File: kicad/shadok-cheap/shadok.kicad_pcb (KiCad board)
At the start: 2 copper layers, 141.2 x 57.8 mm, 123 parts, among them J101 TEST_1P, J103 TEST_1P, J104 TEST_1P, J105 SERIALS, J401 Conn_02x05_Odd_Even, J501 Micro_SD_Card, J502 TEST_1P, J601 74LVC8T245, J602 74LVC8T245, J603 74LVC8T245, J604 SNP34-90, J605 74LVC8T245, J701 DB9_Male_MountingHoles, J702 DB9_Male_MountingHoles, J801 Conn_01x02, J815 Audio Out, SW101 SW_Push, U201 ADP2108-1.2, U202 LP2985-2.5, U203 ADP2108-3.3, U301 IS42S16400J, U501 ESP12F, U601 74LVC1T45, U701 MCP23S17, U801 TPA6110A2, X101 KXO-V97 50MHz

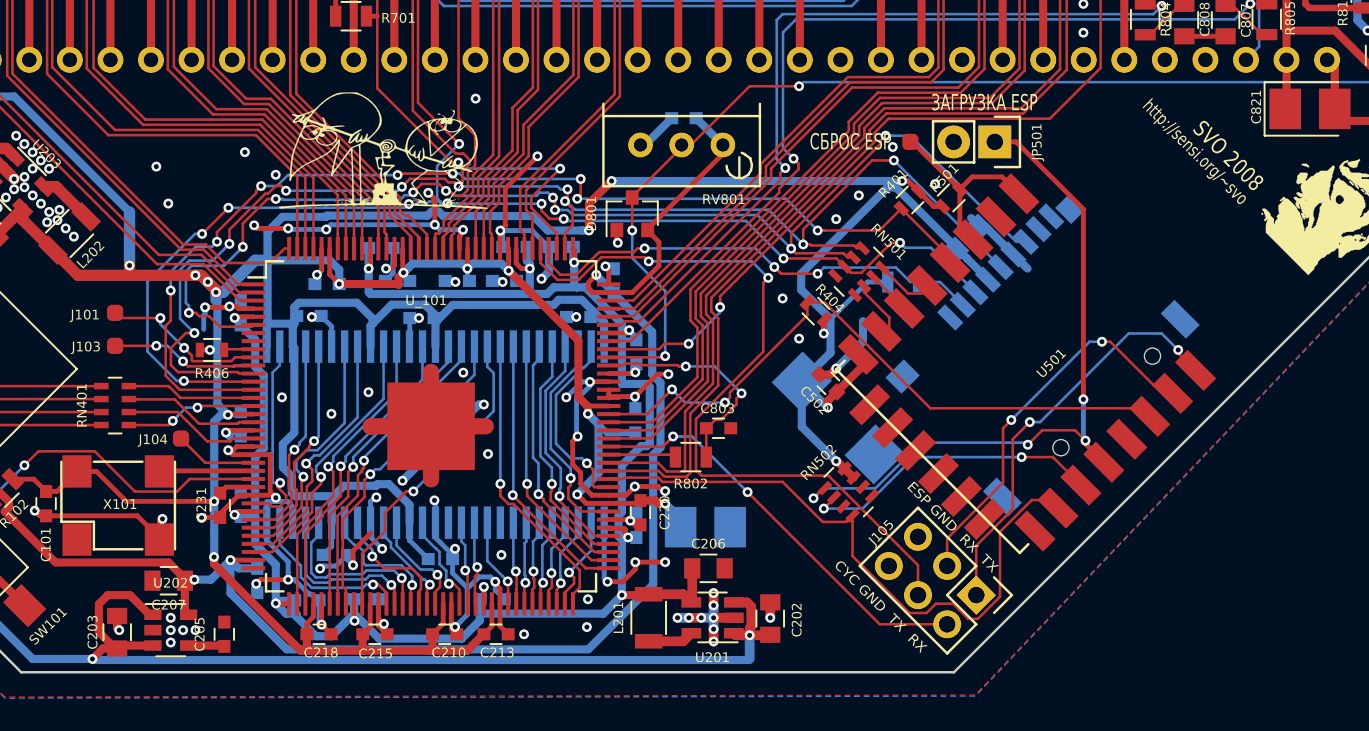
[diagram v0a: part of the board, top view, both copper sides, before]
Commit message: waveforms
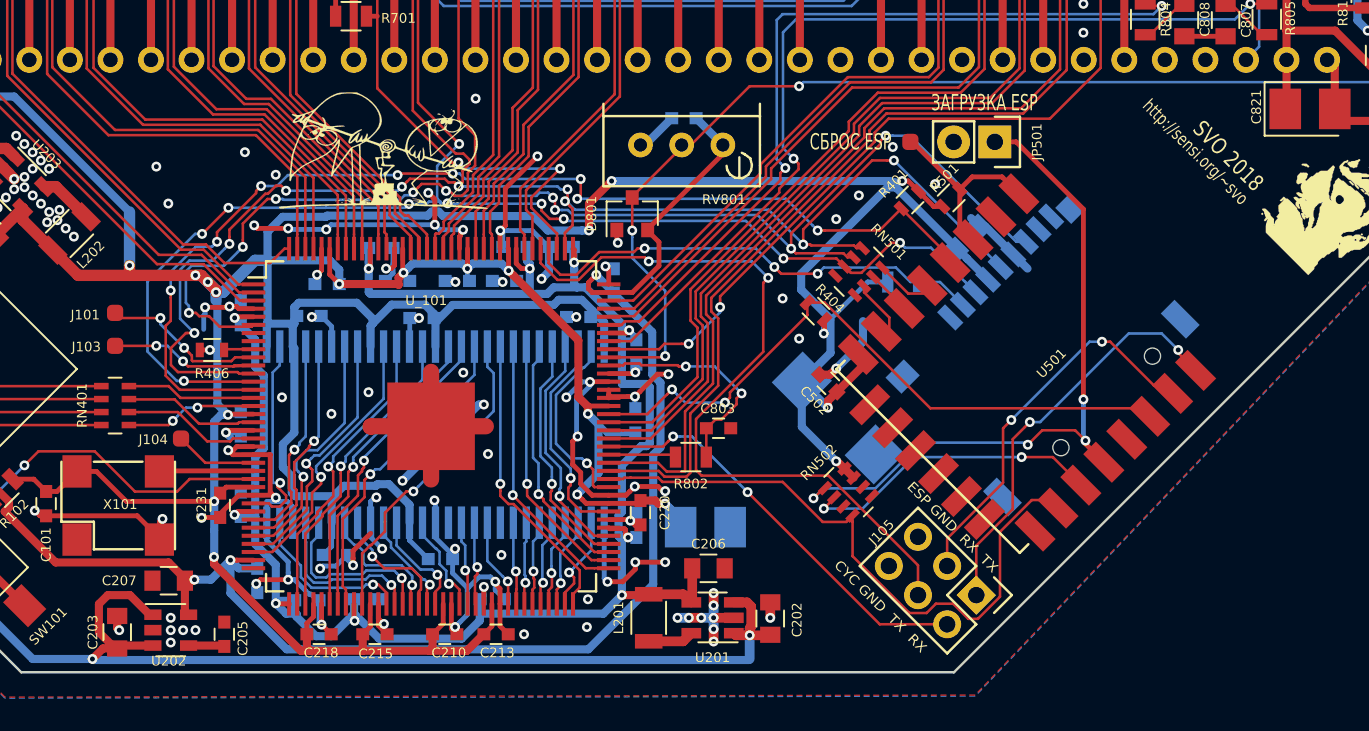
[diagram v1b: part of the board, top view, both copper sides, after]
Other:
- board text added: "SVO 2018"
- board text removed: "SVO 2008"
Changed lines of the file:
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@@
   )
   (setup
-    (last_trace_width 1)
+    (last_trace_width 0.16)
     (user_trace_width 0.3)
     (user_trace_width 0.4)
@@
     (tags "capacitor 0603")
     (attr smd)
-    (fp_text reference C205 (at 0 -1.5 90) (layer F.SilkS)
+    (fp_text reference C205 (at -0.254 1.143 90) (layer F.SilkS)
       (effects (font (size 0.6 0.6) (thickness 0.15)))
     )
@@
     (tags "capacitor 0805")
     (attr smd)
-    (fp_text reference C207 (at 0 -1.5 180) (layer F.SilkS)
+    (fp_text reference C207 (at 3.048 0 180) (layer F.SilkS)
       (effects (font (size 0.6 0.6) (thickness 0.15)))
     )
@@
     (tags SOT-23-5)
     (attr smd)
-    (fp_text reference U202 (at 0 -2.9) (layer F.SilkS)
+    (fp_text reference U202 (at -0.127 1.905) (layer F.SilkS)
       (effects (font (size 0.6 0.6) (thickness 0.15)))
     )
@@
     (effects (font (size 1 1.5) (thickness 0.25)))
   )
-  (gr_text "SVO 2008" (at 160.3375 165.1 315) (layer F.SilkS)
+  (gr_text "SVO 2018" (at 160.3375 165.1 315) (layer F.SilkS)
     (effects (font (size 1 0.8) (thickness 0.15)) (justify right))
   )
